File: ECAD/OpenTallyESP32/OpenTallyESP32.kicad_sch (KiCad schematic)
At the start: 1 part, among them U1 XIAO ESP32C3

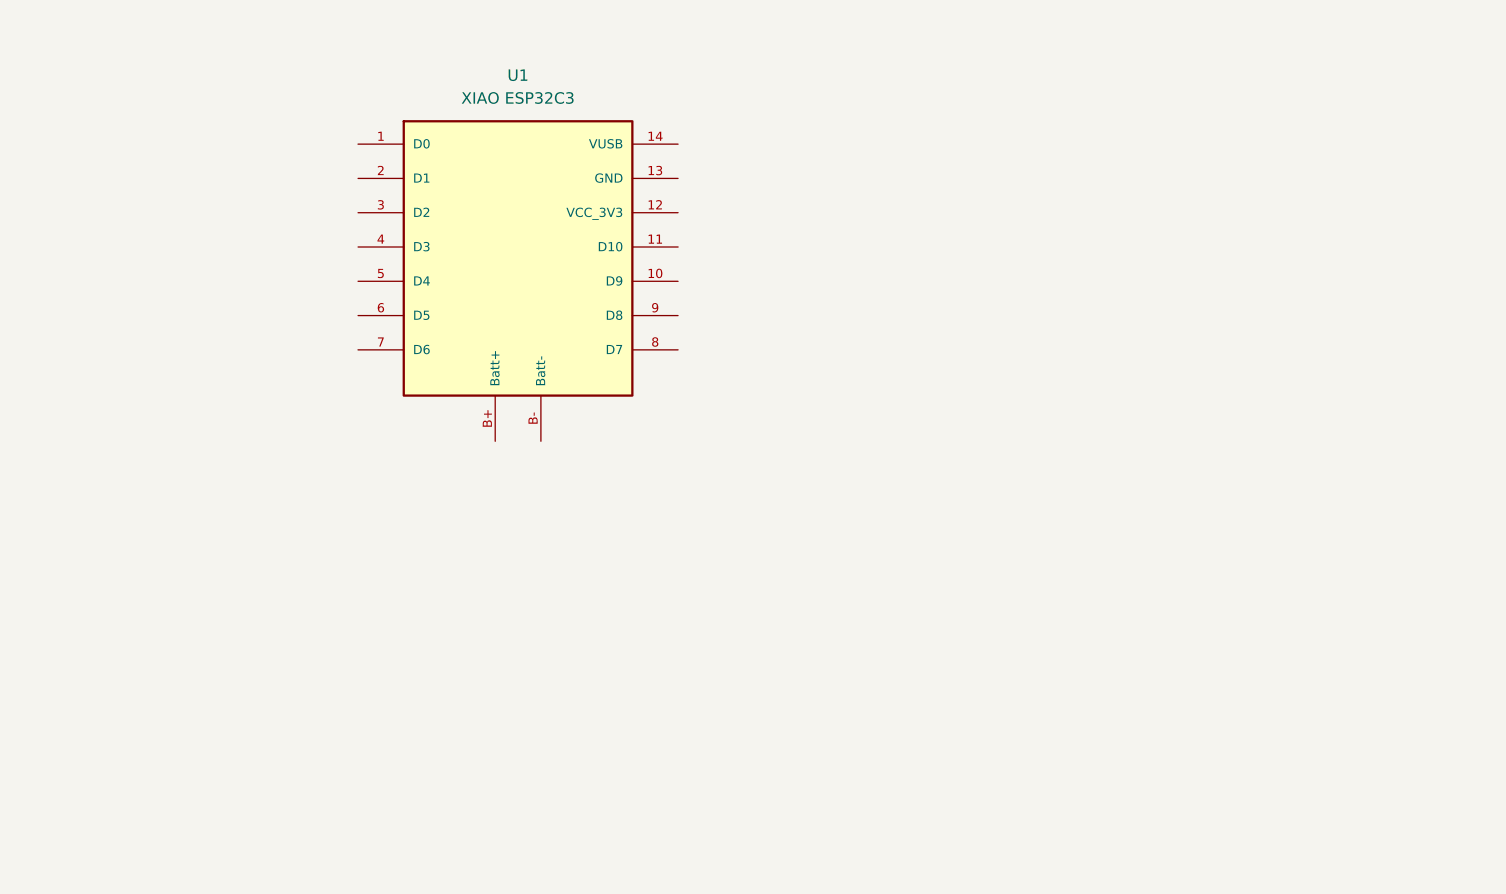
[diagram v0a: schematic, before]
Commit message: Added ESP32
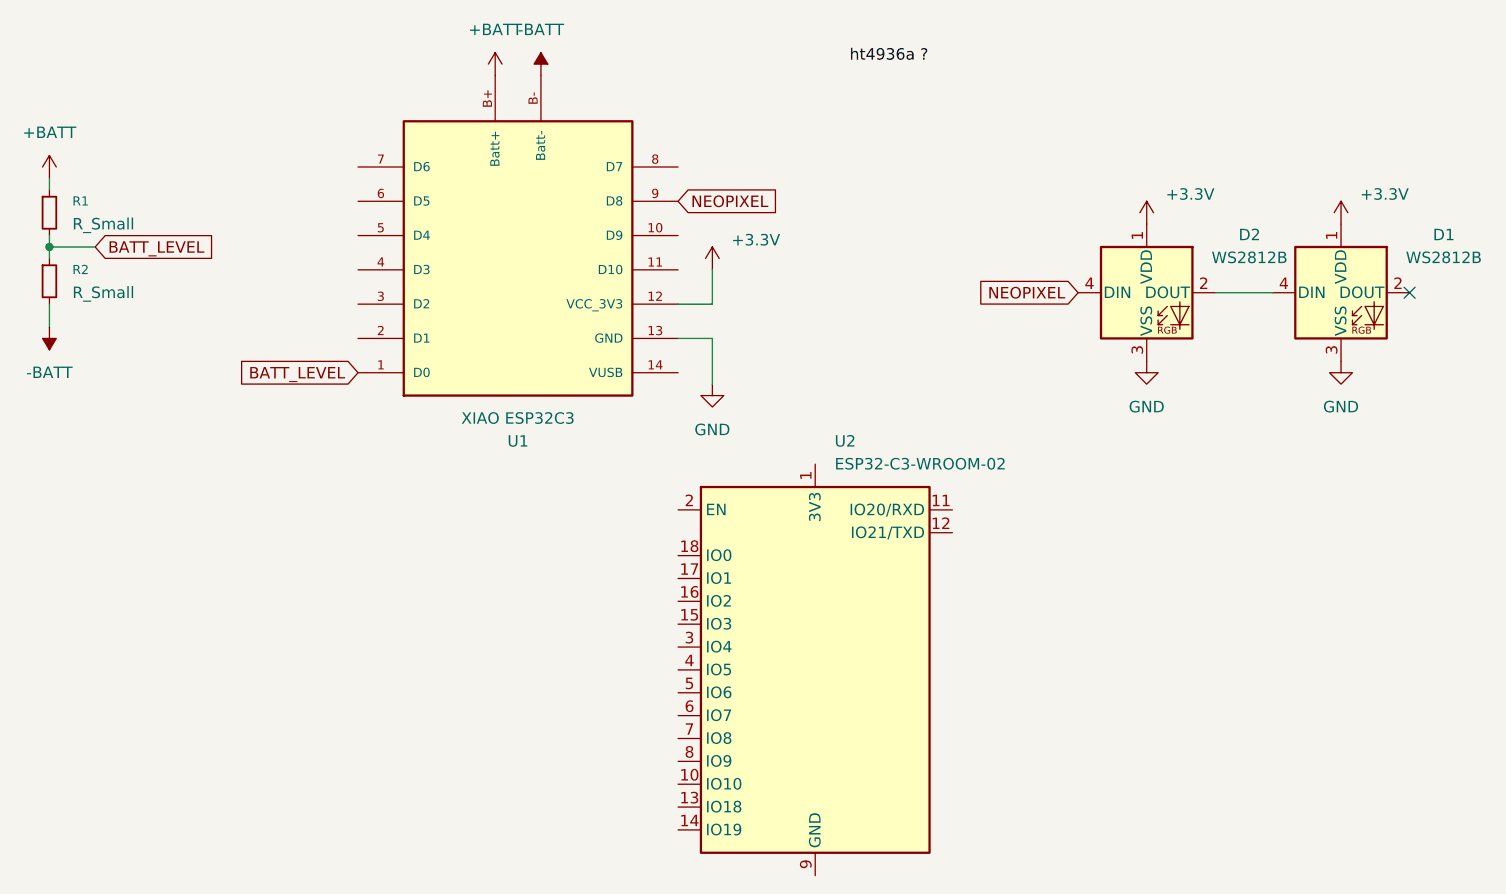
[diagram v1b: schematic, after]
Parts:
- added D1, D2: WS2812B, LED_SMD:LED_WS2812B_PLCC4_5.0x5.0mm_P3.2mm, symbol LED:WS2812B
- added R1, R2: R_Small, symbol Device:R_Small
- added U2: ESP32-C3-WROOM-02, RF_Module:ESP32-C3-WROOM-02, symbol RF_Module:ESP32-C3-WROOM-02
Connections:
- net BATT_LEVEL: now reaches U1.1 (D0)
- net BATT_LEVEL: now also R1.2, R2.1
- net +3.3V: now reaches U1.12 (VCC_3V3)
- net +3.3V: now also D1.1 (VDD), D2.1 (VDD)
- net GND: now reaches U1.13 (GND)
- net GND: now also D1.3 (VSS), D2.3 (VSS)
- net NEOPIXEL: now reaches U1.9 (D8)
- net NEOPIXEL: now also D2.4 (DIN)
- net +BATT: now reaches U1.B+ (Batt+)
- net +BATT: now also R1.1
- net -BATT: now reaches U1.B- (Batt-)
- net -BATT: now also R2.2
- new net: D1.4 (DIN), D2.2 (DOUT)
- new net: U2.19 (GND), U2.9 (GND)
- no-connect marks 0 -> 1
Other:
- moved on the sheet: U1
